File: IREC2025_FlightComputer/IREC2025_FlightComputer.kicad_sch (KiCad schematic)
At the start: 67 parts, among them J1 Molex Microfit, J2 BOOT0, J3 Companion, J5 SWD, Q1 SI7232DN-T1-GE3, U1 STM32U575VGTx, U2 NRVB120VLSFT1G, U4 NRVB120VLSFT1G, U5 LP5912Q3.3DRVRQ1, U8 TPS62153, U9 SN74HCT125DR, X1 1XXD32000MBA

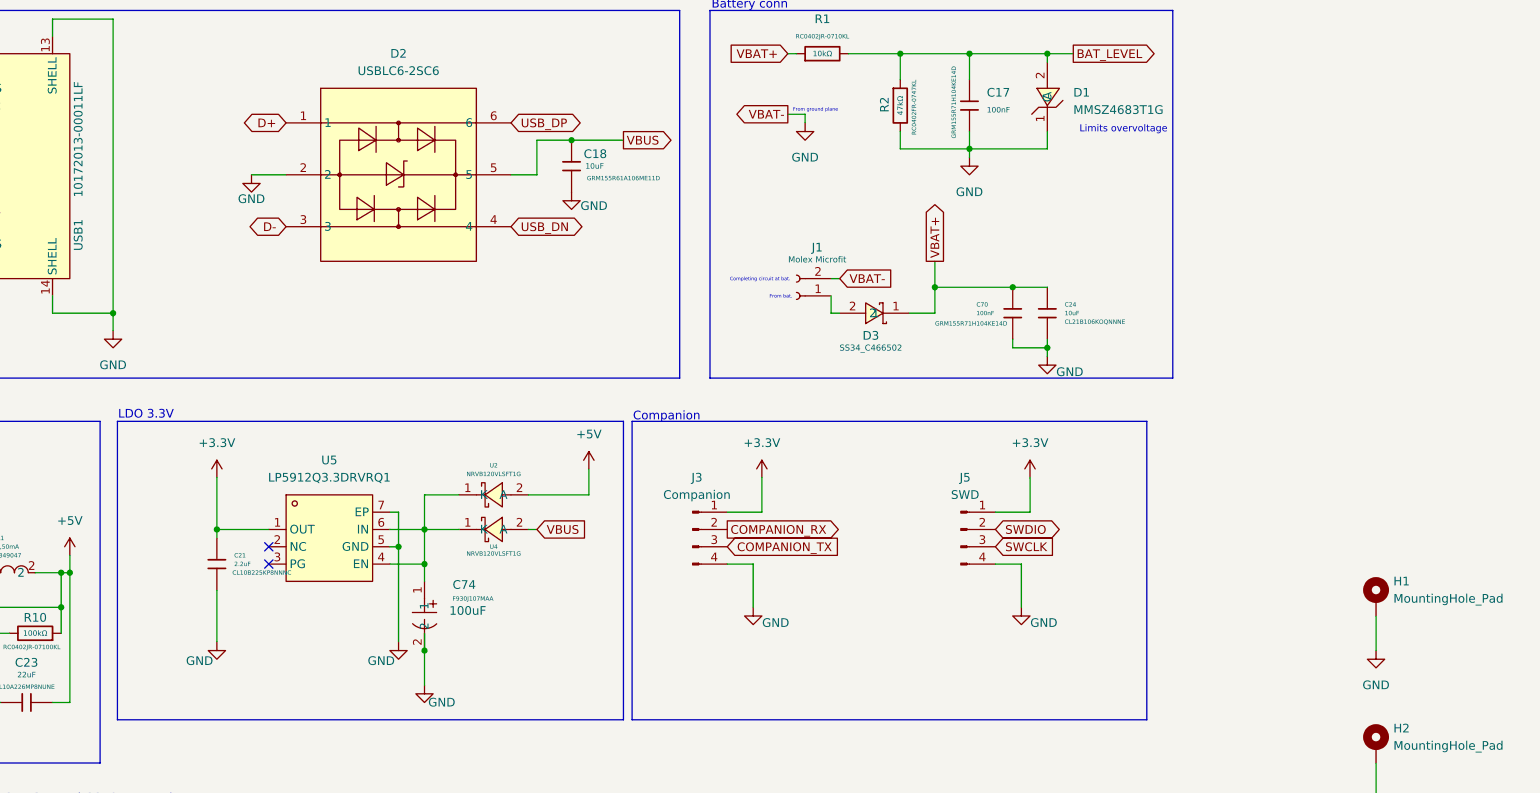
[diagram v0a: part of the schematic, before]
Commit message: small fixes
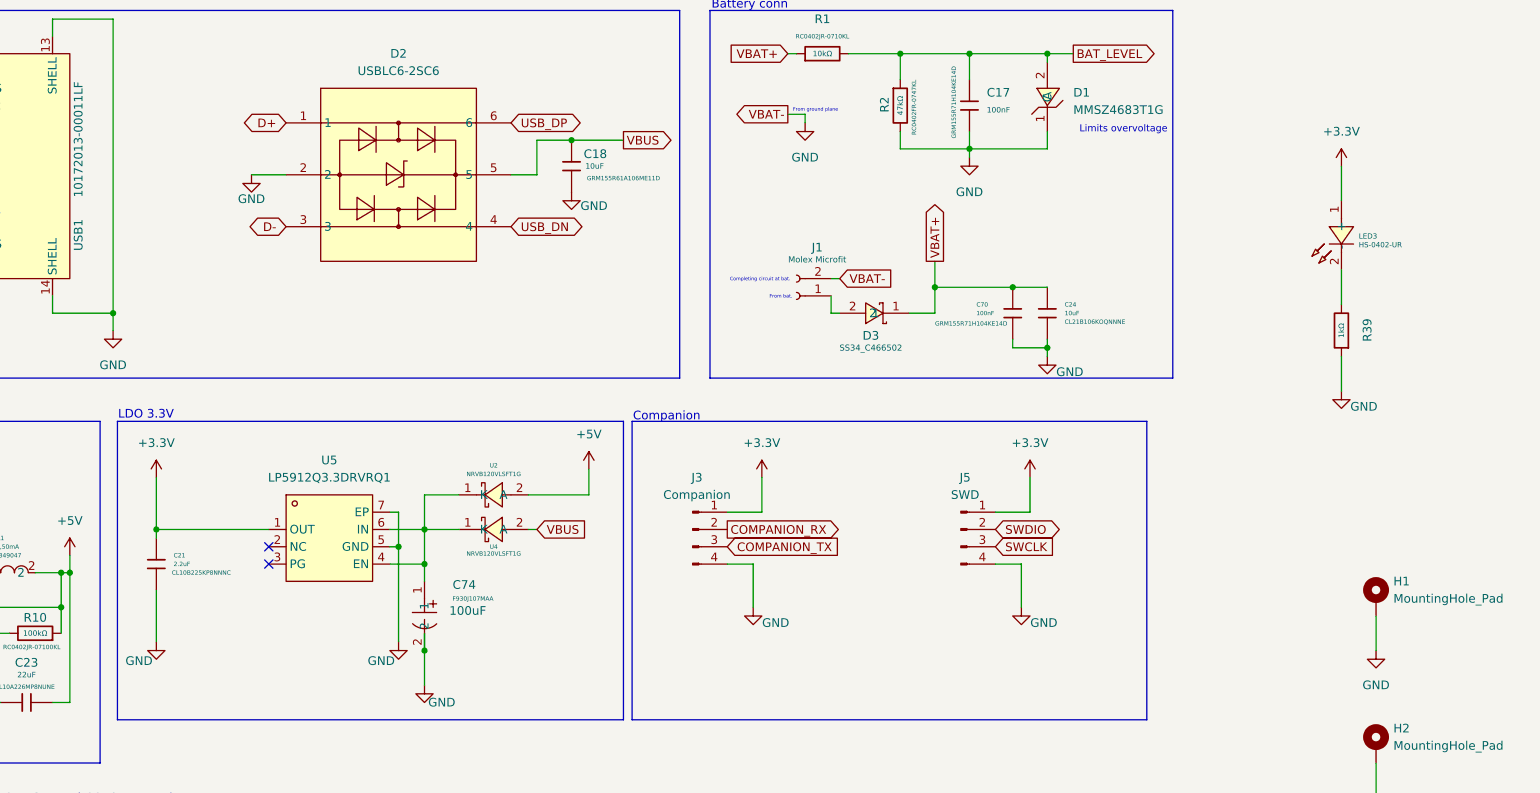
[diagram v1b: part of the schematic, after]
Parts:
- added LED3: HS-0402-UR, EasyEDA:LED0402-R-RD, symbol EasyEDA:HS-0402-UR
- added R39: 1kΩ, PCM_JLCPCB:R_0402, symbol PCM_JLCPCB-Resistors:0402,1kΩ
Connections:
- net +3.3V: now also LED3.1 (+)
- net GND: now also R39.1
- new net: LED3.2 (-), R39.2
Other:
- moved on the sheet: C21
